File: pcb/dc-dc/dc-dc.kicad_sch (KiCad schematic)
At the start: 3 parts, among them U2 LM2595S-3.3

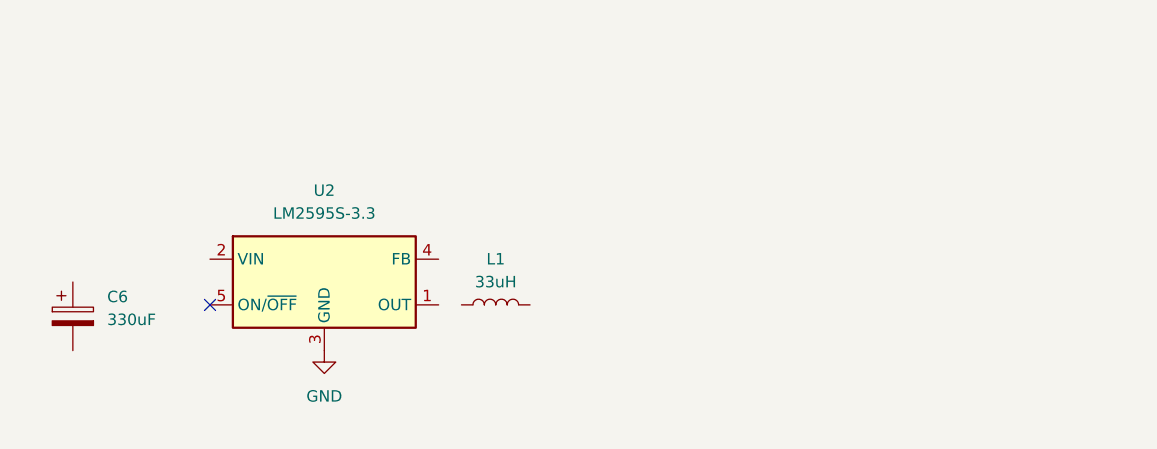
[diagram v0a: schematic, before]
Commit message: update
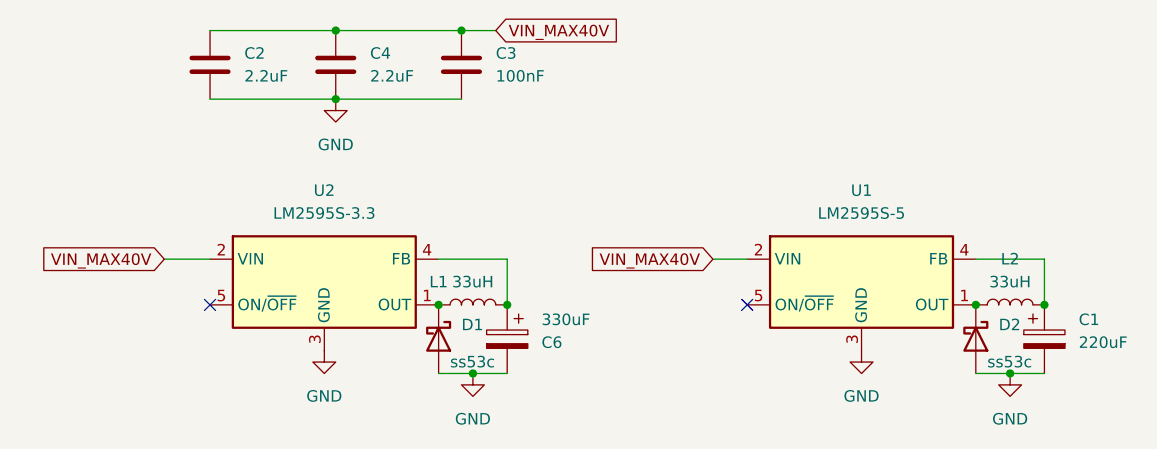
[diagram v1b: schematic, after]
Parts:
- added C1: 220uF, symbol Device:C_Polarized
- added C2, C4: 2.2uF, symbol Device:C
- added C3: 100nF, symbol Device:C
- added D1, D2: ss53c, symbol Device:D_Schottky
- added L2: 33uH, symbol Device:L
- added U1: LM2595S-5, Package_TO_SOT_SMD:TO-263-5_TabPin3, symbol Regulator_Switching:LM2595S-5
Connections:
- net GND: now also C6.2, C1.2, C2.1, C3.1, C4.1, D1.2 (A), D2.2 (A), U1.3 (GND)
- net at C6.1: now also L1.2, U2.4 (FB)
- net at L1.1: now also U2.1 (OUT), D1.1 (K)
- net VIN_MAX40V: now reaches U2.2 (VIN)
- net VIN_MAX40V: now also C2.2, C3.2, C4.2, U1.2 (VIN)
- new net: D2.1 (K), L2.1, U1.1 (OUT)
- new net: C1.1, L2.2, U1.4 (FB)
- no-connect marks 1 -> 2
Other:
- moved on the sheet: C6, L1

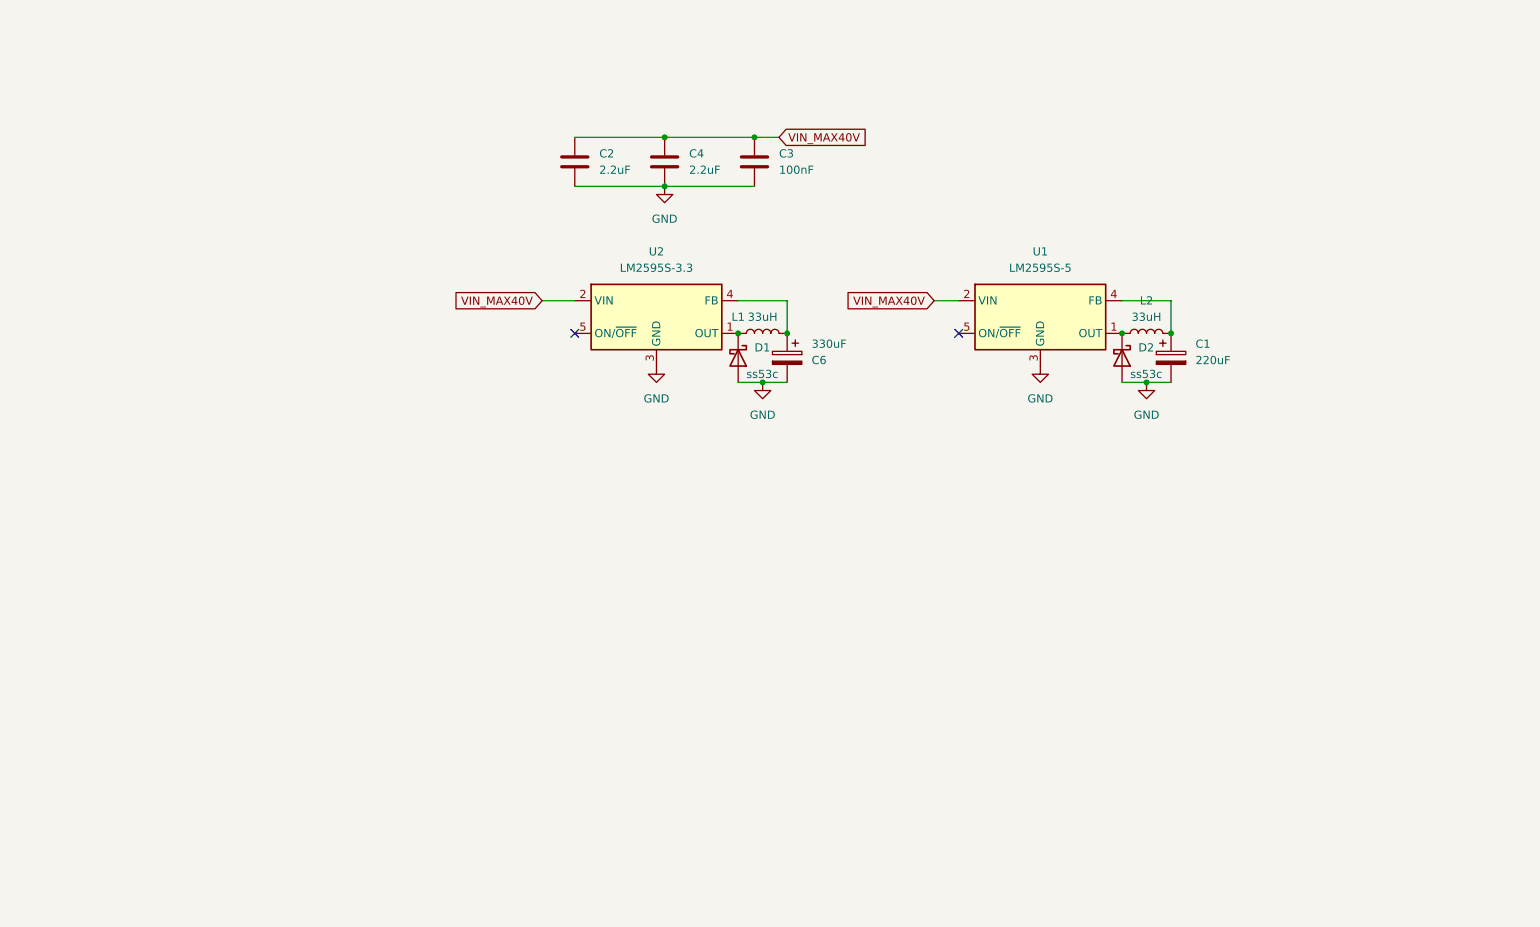
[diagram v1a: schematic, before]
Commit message: feat: update
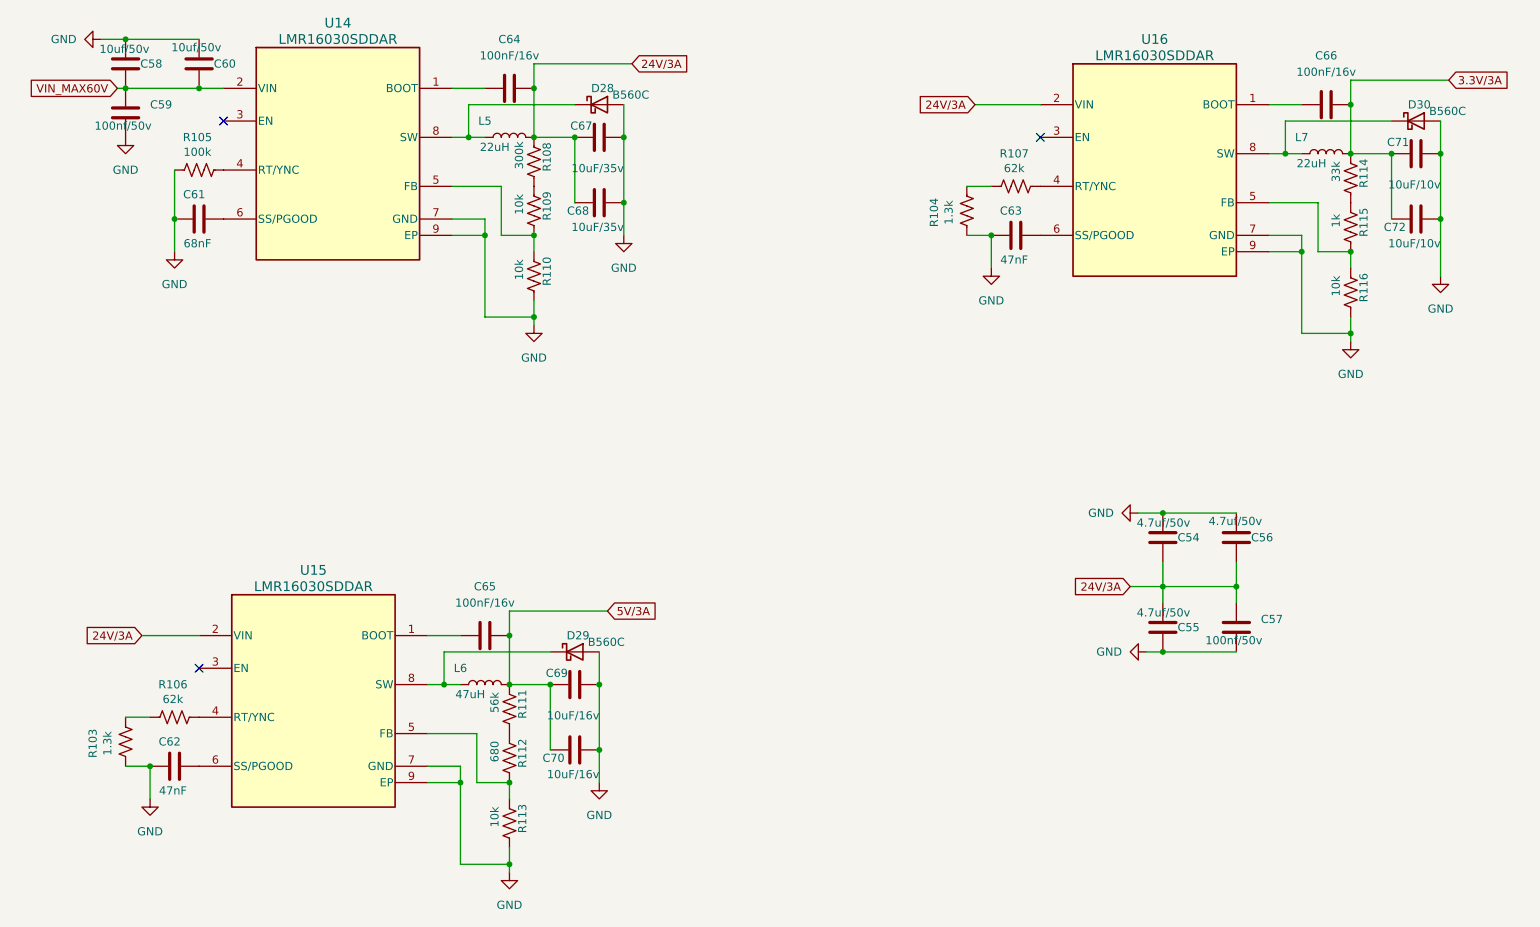
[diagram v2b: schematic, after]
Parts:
- removed C1: 220uF, symbol Device:C_Polarized
- removed C2, C4: 2.2uF, symbol Device:C
- removed C3: 100nF, symbol Device:C
- removed C6: 330uF, symbol Device:C_Polarized
- removed D1, D2: ss53c, symbol Device:D_Schottky
- removed L1, L2: 33uH, symbol Device:L
- removed U1: LM2595S-5, Package_TO_SOT_SMD:TO-263-5_TabPin3, symbol Regulator_Switching:LM2595S-5
- removed U2: LM2595S-3.3, Package_TO_SOT_SMD:TO-263-5_TabPin3, symbol Regulator_Switching:LM2595S-3.3
- added C54, C55, C56: 4.7uf/50v, Capacitor_SMD:C_1206_3216Metric, symbol Device:C
- added C57, C59: 100nf/50v, Capacitor_SMD:C_0603_1608Metric, symbol Device:C
- added C58, C60: 10uf/50v, Capacitor_SMD:C_1210_3225Metric, symbol Device:C
- added C61: 68nF, Capacitor_SMD:C_0603_1608Metric, symbol Device:C
- added C62, C63: 47nF, Capacitor_SMD:C_0603_1608Metric, symbol Device:C
- added C64, C65, C66: 100nF/16v, Capacitor_SMD:C_0603_1608Metric, symbol Device:C
- added C67, C68: 10uF/35v, Capacitor_SMD:C_1210_3225Metric, symbol Device:C
- added C69, C70: 10uF/16v, Capacitor_SMD:C_1210_3225Metric, symbol Device:C
- added C71, C72: 10uF/10v, Capacitor_SMD:C_0603_1608Metric, symbol Device:C
- added D28, D29, D30: B560C, Diode_SMD:D_SMC, symbol Device:D_Schottky
- added L5, L7: 22uH, Inductor_SMD:L_TDK_SLF12565, symbol Device:L
- added L6: 47uH, Inductor_SMD:L_TDK_SLF12565, symbol Device:L
- added R103, R104: 1.3k, Resistor_SMD:R_0603_1608Metric, symbol Device:R_US
- added R105: 100k, Resistor_SMD:R_0603_1608Metric, symbol Device:R_US
- added R106, R107: 62k, Resistor_SMD:R_0603_1608Metric, symbol Device:R_US
- added R108: 300k, Resistor_SMD:R_0603_1608Metric, symbol Device:R_US
- added R109, R110, R113, R116: 10k, Resistor_SMD:R_0603_1608Metric, symbol Device:R_US
- added R111: 56k, Resistor_SMD:R_0603_1608Metric, symbol Device:R_US
- added R112: 680, Resistor_SMD:R_0603_1608Metric, symbol Device:R_US
- added R114: 33k, Resistor_SMD:R_0603_1608Metric, symbol Device:R_US
- added R115: 1k, Resistor_SMD:R_0603_1608Metric, symbol Device:R_US
- added U14, U15, U16: LMR16030SDDAR, Package_SO:TI_SO-PowerPAD-8_ThermalVias, symbol 2025-01-08_11-11-09:LMR16030SDDAR
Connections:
- net GND: now also C54.2, C55.1, C56.1, C57.2, C58.2, C59.2, C60.1, C61.2, C62.2, C63.2, C67.2, C68.1, C69.2, C70.1, C71.2, C72.1, D28.2 (A), D29.2 (A), D30.2 (A), R103.2, R104.2, R105.2, R110.2, R113.2, R116.2, U14.7 (GND), U14.9 (EP), U15.7 (GND), U15.9 (EP), U16.7 (GND), U16.9 (EP)
- new net: C62.1, U15.6 (SS/PGOOD)
- new net: D28.1 (K), L5.1, U14.8 (SW)
- new net: C66.2, U16.1 (BOOT)
- new net: R107.1, U16.4 (RT/YNC)
- new net: R115.2, R116.1, U16.5 (FB)
- new net: C63.1, U16.6 (SS/PGOOD)
- new net: D30.1 (K), L7.1, U16.8 (SW)
- new net: R108.2, R109.1
- new net: C64.2, U14.1 (BOOT)
- new net: R105.1, U14.4 (RT/YNC)
- new net: R109.2, R110.1, U14.5 (FB)
- new net: C61.1, U14.6 (SS/PGOOD)
- new net: C65.2, U15.1 (BOOT)
- new net: R103.1, R106.2
- new net: R112.2, R113.1, U15.5 (FB)
- new net: D29.1 (K), L6.1, U15.8 (SW)
- new net: R106.1, U15.4 (RT/YNC)
- new net: R104.1, R107.2
- new net: R114.2, R115.1
- new net: R111.2, R112.1
- new net 24V/3A: C54.1, C55.2, C56.2, C57.1, C64.1, C67.1, C68.2, L5.2, R108.1, U15.2 (VIN), U16.2 (VIN)
- new net 3.3V/3A: C66.1, C71.1, C72.2, L7.2, R114.1
- new net 5V/3A: C65.1, C69.1, C70.2, L6.2, R111.1
- new net VIN_MAX60V: C58.1, C59.1, C60.2, U14.2 (VIN)
- no-connect marks 2 -> 3
